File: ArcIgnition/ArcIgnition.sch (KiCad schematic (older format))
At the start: 7 parts

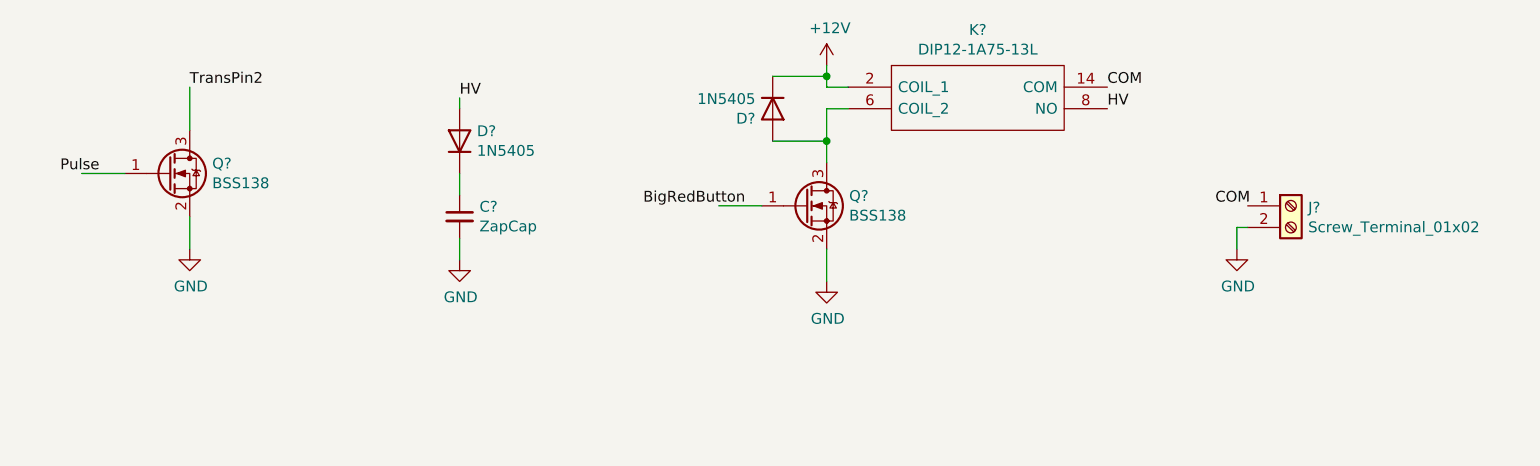
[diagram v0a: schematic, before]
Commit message: Fixing the mistakes as always
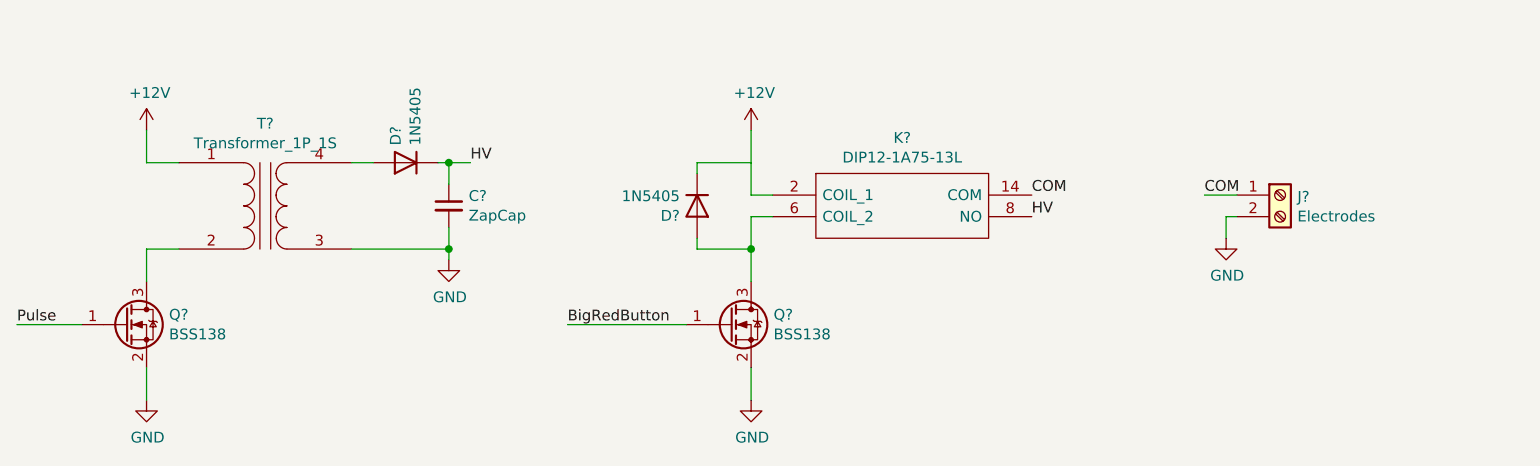
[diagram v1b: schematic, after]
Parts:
- added T?: Transformer_1P_1S, symbol Device:Transformer_1P_1S
- J?: value Screw_Terminal_01x02 -> Electrodes
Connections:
- net labels removed: TransPin2
- wire segments 18 -> 28
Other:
- moved on the sheet: C?, D?, J?, K?, Q?
